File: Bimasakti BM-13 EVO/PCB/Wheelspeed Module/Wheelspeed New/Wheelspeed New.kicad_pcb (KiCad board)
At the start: 2 copper layers, 32 x 46.5 mm, 21 parts, among them J3 Conn_01x15_Pin, J4 Conn_01x15_Pin, U1 ESP32-C3_SUPERMINI_TH, U2 LM393

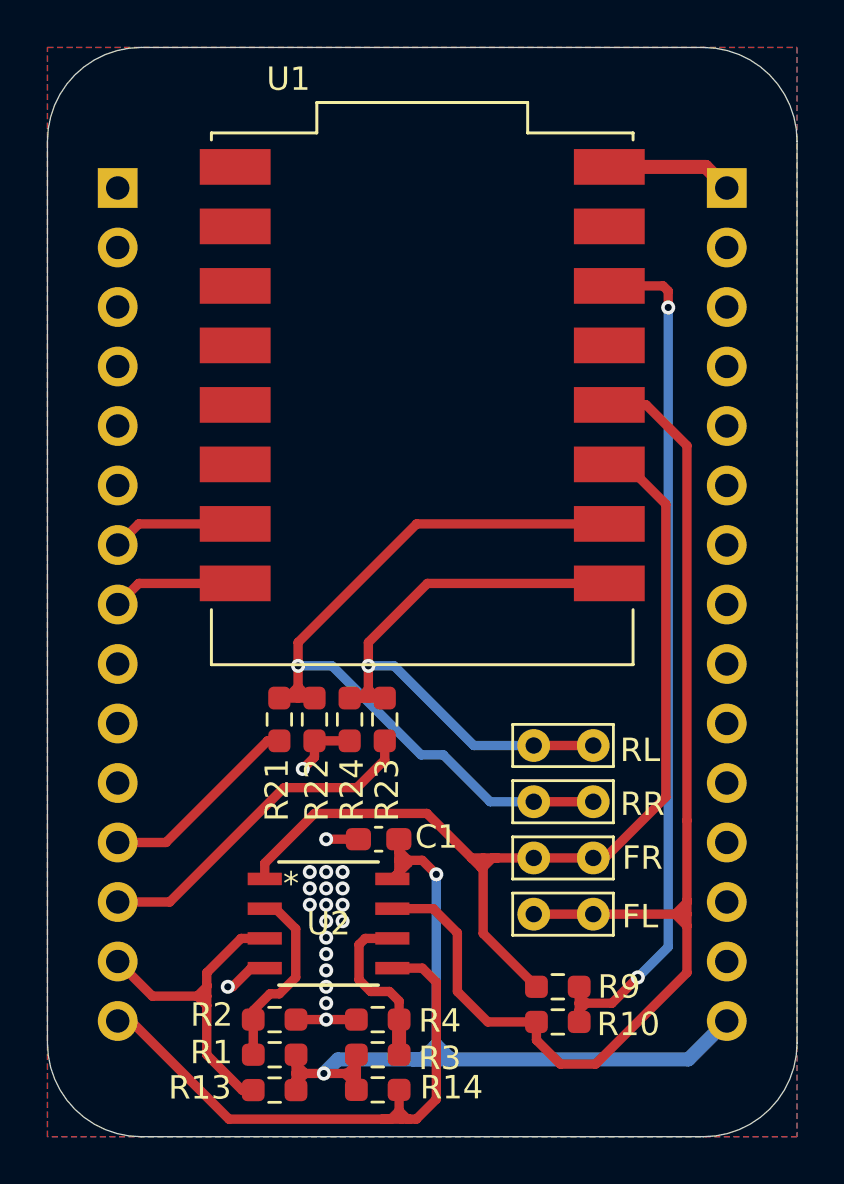
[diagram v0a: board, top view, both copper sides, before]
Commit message: tv board FIXXXXX
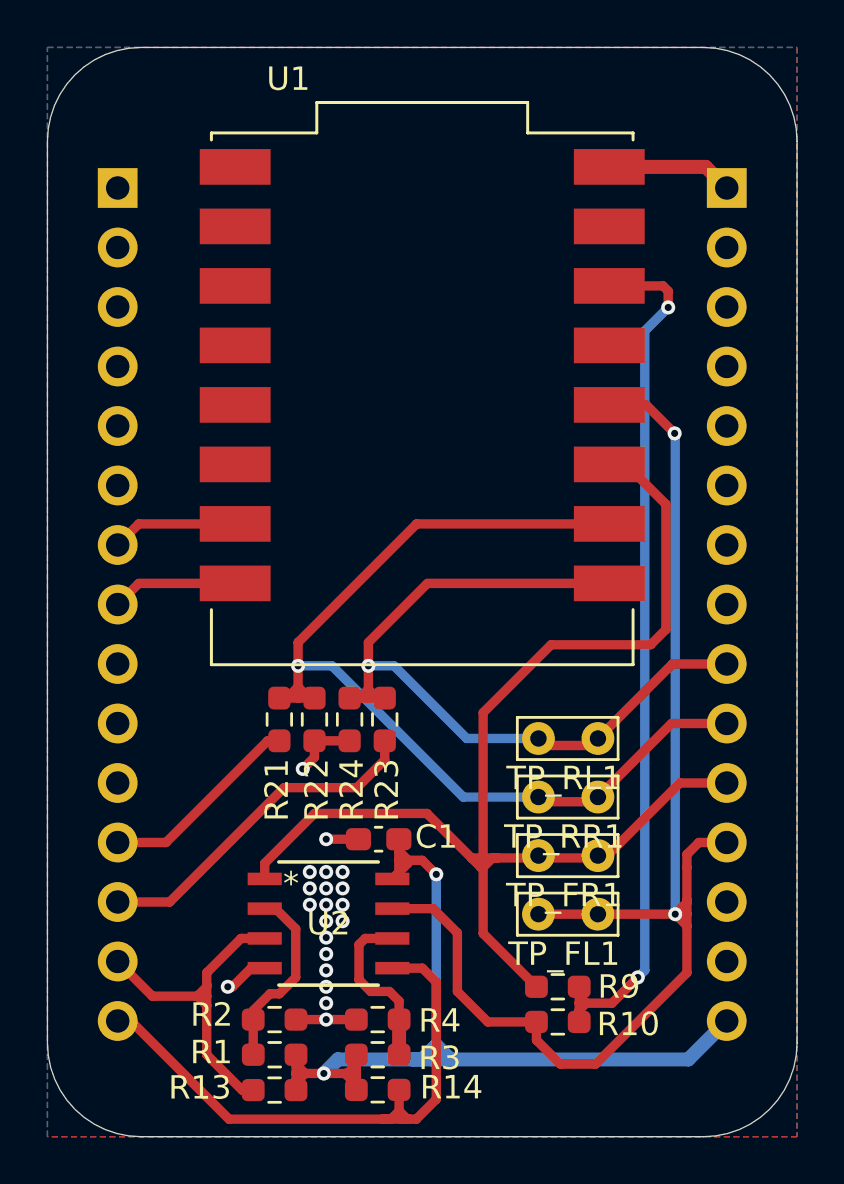
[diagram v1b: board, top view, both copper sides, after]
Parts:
- removed FL, FR, RL, RR: TestPoint, TestPoint:TestPoint_Bridge_Pitch2.54mm_Drill0.7mm
- added TP_FL1: TestPoint, TestPoint:TestPoint_Bridge_Pitch2.54mm_Drill0.7mm, F.Cu at (120.0, 139.0)
- added TP_FR1: TestPoint, TestPoint:TestPoint_Bridge_Pitch2.54mm_Drill0.7mm, F.Cu at (120.0, 136.5)
- added TP_RL1: TestPoint, TestPoint:TestPoint_Bridge_Pitch2.54mm_Drill0.7mm, F.Cu at (120.0, 131.5)
- added TP_RR1: TestPoint, TestPoint:TestPoint_Bridge_Pitch2.54mm_Drill0.7mm, F.Cu at (120.0, 134.0)
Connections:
- J4 pad 10: unconnected-(J4-Pin_10-Pad10) -> /WS_RR_Signal
- J4 pad 11: unconnected-(J4-Pin_11-Pad11) -> /WS_FR_Signal
- J4 pad 12: unconnected-(J4-Pin_12-Pad12) -> /WS_FL_Signal
- J4 pad 9: unconnected-(J4-Pin_9-Pad9) -> /WS_RL_Signal
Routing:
- net /WS_FR_Signal: track 44.0 -> 55.2 mm
- net /WS_RR_Signal: track 36.9 -> 43.8 mm
- net /WS_RL_Signal: track 29.1 -> 36.0 mm
- net /WS_FL_Signal: track 53.4 -> 57.7 mm, vias 0 -> 2
